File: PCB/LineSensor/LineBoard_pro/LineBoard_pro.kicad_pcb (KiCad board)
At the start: 2 copper layers, 20 parts, among them IC1 NJL7502R, IC2 NJL7502R, IC3 NJL7502R, IC4 NJL7502R, J1 to MAIN, U1 TMUX1204DGSR

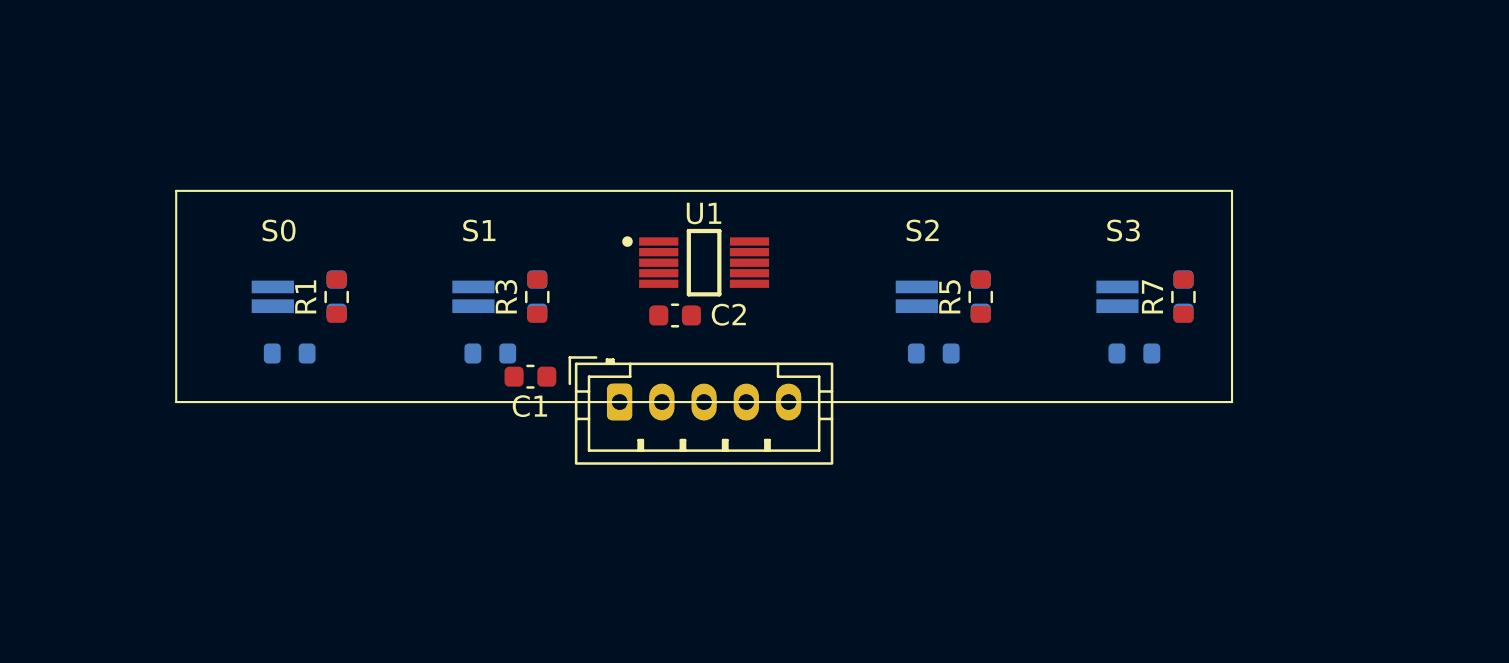
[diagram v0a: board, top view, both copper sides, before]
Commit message: ラインセンサ完成
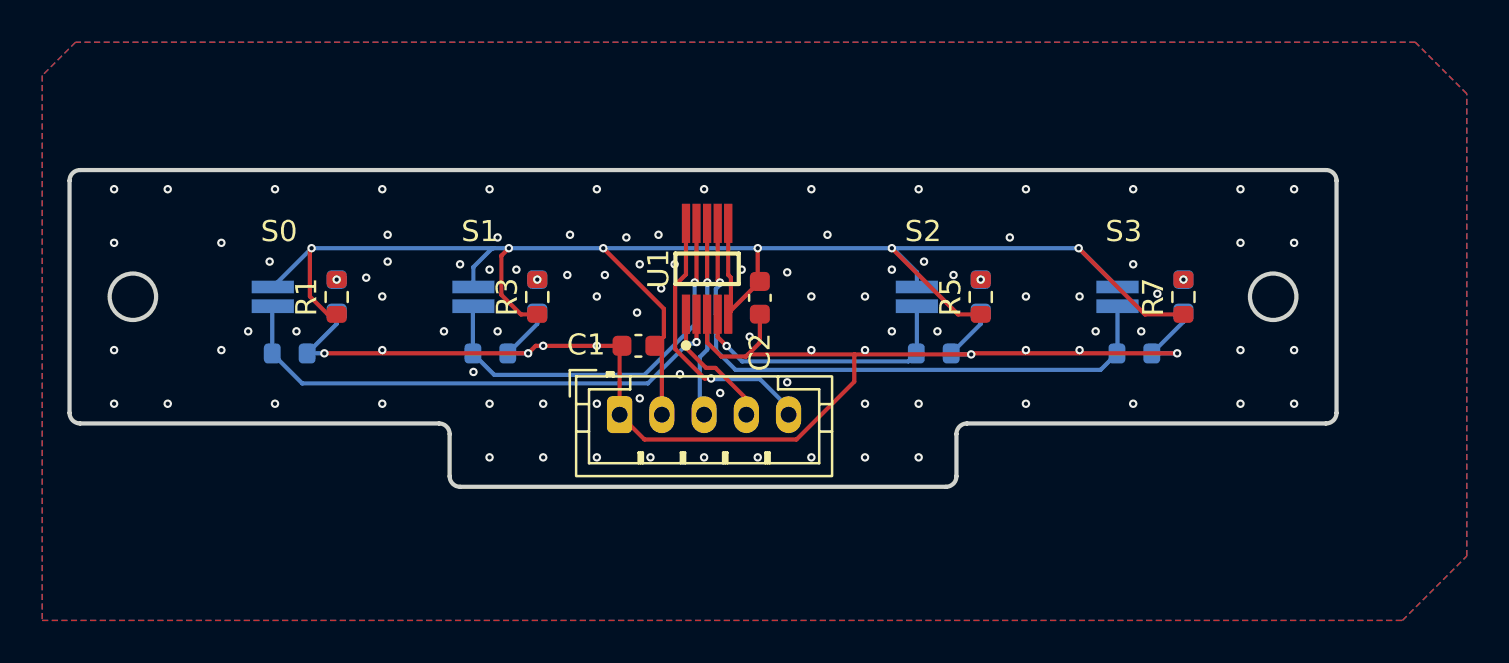
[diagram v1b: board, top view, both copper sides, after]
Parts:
- moved C1 5.32 mm to (96.9, 37.3)
- moved C2 4.10 mm to (102.6, 35.1), turned to -90 degrees
- moved J1 0.60 mm to (96.0, 40.6)
- moved U1 0.32 mm to (100.1, 33.7), turned to 90 degrees
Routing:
- net +3V3: track 0.00 -> 83.9 mm, vias 0 -> 6
- net GND: track 0.00 -> 71.8 mm, vias 0 -> 100
- net /S3: track 0.00 -> 28.1 mm, vias 0 -> 1
- net /S0: track 0.00 -> 25.1 mm, vias 0 -> 1
- net /S1: track 0.00 -> 19.0 mm, vias 0 -> 1
- net /S2: track 0.00 -> 13.4 mm, vias 0 -> 1
- net /Line_A1: track 0.00 -> 13.0 mm, vias 0 -> 1
- net /Line_OUT: track 0.00 -> 9.29 mm, vias 0 -> 1
- net /Line_A0: track 0.00 -> 6.20 mm
- net Net-(D4-A): vias 0 -> 1
- net Net-(D3-A): vias 0 -> 1
- net Net-(D2-A): vias 0 -> 1
- net Net-(D1-A): vias 0 -> 1
- added copper zone on B.Cu, net GND
- added copper zone on F.Cu, net GND
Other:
- board outline added: 60 x 15 mm
